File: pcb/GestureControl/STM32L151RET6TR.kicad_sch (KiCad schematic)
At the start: 33 parts, among them J10 EXTERN I2C, J11 Conn_01x02, J12 Conn_01x02, J17 Conn_01x01, J18 Conn_01x01, J19 Conn_01x01, J7 FTDI, J8 Conn_01x06, J9 UART, U6 STM32L151RETx, U7 STM32F401RETx, Y1 8MHz, Y2 32kHz

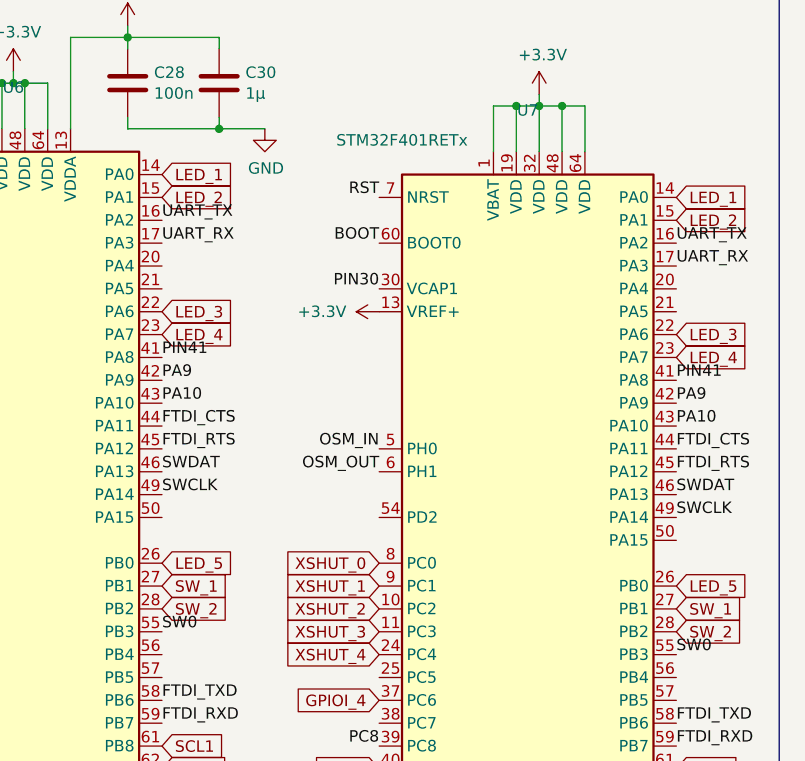
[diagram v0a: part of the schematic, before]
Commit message: add docs
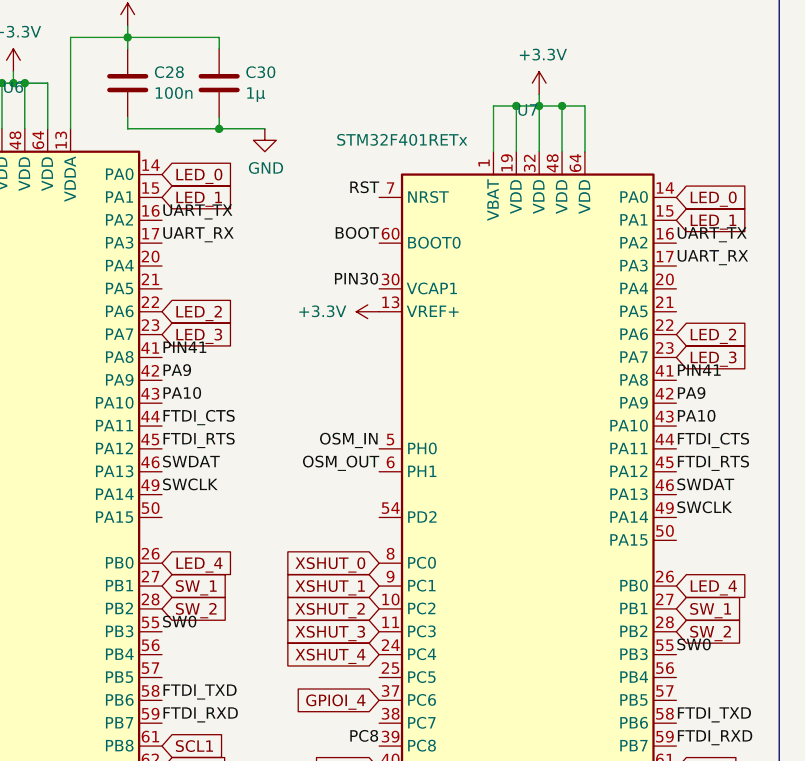
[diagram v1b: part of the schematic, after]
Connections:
- net LED_5 is gone; now on net LED_4: U6.26 (PB0), U7.26 (PB0)
- net LED_1: now also U6.15 (PA1), U7.15 (PA1); no longer U6.14 (PA0), U7.14 (PA0)
- net LED_2: now also U6.22 (PA6), U7.22 (PA6); no longer U6.15 (PA1), U7.15 (PA1)
- net LED_3: now also U6.23 (PA7), U7.23 (PA7); no longer U6.22 (PA6), U7.22 (PA6)
- net LED_4: no longer U6.23 (PA7), U7.23 (PA7)
- new net LED_0: U6.14 (PA0), U7.14 (PA0)
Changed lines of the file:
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@@
     )
   )
-  (global_label "LED_4" (shape input) (at 250.19 60.96 0) (fields_autoplaced)
-    (effects (font (size 1.27 1.27)) (justify left))
-    (property "Intersheet References" "${INTERSHEET_REFS}" (id 0) (at 0 0 0)
-      (effects (font (size 1.27 1.27)) hide)
-    )
-  )
-  (global_label "LED_1" (shape input) (at 193.04 40.64 0) (fields_autoplaced)
-    (effects (font (size 1.27 1.27)) (justify left))
-    (property "Intersheet References" "${INTERSHEET_REFS}" (id 0) (at 0 0 0)
-      (effects (font (size 1.27 1.27)) hide)
+  (global_label "LED_3" (shape input) (at 250.19 60.96 0) (fields_autoplaced)
+    (effects (font (size 1.27 1.27)) (justify left))
+    (property "Intersheet References" "${INTERSHEET_REFS}" (id 0) (at 258.1385 60.8806 0)
+      (effects (font (size 1.27 1.27)) (justify left) hide)
+    )
+  )
+  (global_label "LED_0" (shape input) (at 193.04 40.64 0) (fields_autoplaced)
+    (effects (font (size 1.27 1.27)) (justify left))
+    (property "Intersheet References" "${INTERSHEET_REFS}" (id 0) (at 200.9885 40.5606 0)
+      (effects (font (size 1.27 1.27)) (justify left) hide)
     )
   )
@@
     )
   )
-  (global_label "LED_2" (shape input) (at 193.04 43.18 0) (fields_autoplaced)
-    (effects (font (size 1.27 1.27)) (justify left))
-    (property "Intersheet References" "${INTERSHEET_REFS}" (id 0) (at 0 0 0)
-      (effects (font (size 1.27 1.27)) hide)
+  (global_label "LED_1" (shape input) (at 193.04 43.18 0) (fields_autoplaced)
+    (effects (font (size 1.27 1.27)) (justify left))
+    (property "Intersheet References" "${INTERSHEET_REFS}" (id 0) (at 200.9885 43.1006 0)
+      (effects (font (size 1.27 1.27)) (justify left) hide)
     )
   )
@@
     )
   )
-  (global_label "LED_2" (shape input) (at 250.19 45.72 0) (fields_autoplaced)
-    (effects (font (size 1.27 1.27)) (justify left))
-    (property "Intersheet References" "${INTERSHEET_REFS}" (id 0) (at 0 0 0)
-      (effects (font (size 1.27 1.27)) hide)
-    )
-  )
-  (global_label "LED_3" (shape input) (at 250.19 58.42 0) (fields_autoplaced)
-    (effects (font (size 1.27 1.27)) (justify left))
-    (property "Intersheet References" "${INTERSHEET_REFS}" (id 0) (at 0 0 0)
-      (effects (font (size 1.27 1.27)) hide)
+  (global_label "LED_1" (shape input) (at 250.19 45.72 0) (fields_autoplaced)
+    (effects (font (size 1.27 1.27)) (justify left))
+    (property "Intersheet References" "${INTERSHEET_REFS}" (id 0) (at 258.1385 45.6406 0)
+      (effects (font (size 1.27 1.27)) (justify left) hide)
+    )
+  )
+  (global_label "LED_2" (shape input) (at 250.19 58.42 0) (fields_autoplaced)
+    (effects (font (size 1.27 1.27)) (justify left))
+    (property "Intersheet References" "${INTERSHEET_REFS}" (id 0) (at 258.1385 58.3406 0)
+      (effects (font (size 1.27 1.27)) (justify left) hide)
     )
   )
@@
     )
   )
-  (global_label "LED_1" (shape input) (at 250.19 43.18 0) (fields_autoplaced)
-    (effects (font (size 1.27 1.27)) (justify left))
-    (property "Intersheet References" "${INTERSHEET_REFS}" (id 0) (at 0 0 0)
-      (effects (font (size 1.27 1.27)) hide)
+  (global_label "LED_0" (shape input) (at 250.19 43.18 0) (fields_autoplaced)
+    (effects (font (size 1.27 1.27)) (justify left))
+    (property "Intersheet References" "${INTERSHEET_REFS}" (id 0) (at 258.1385 43.1006 0)
+      (effects (font (size 1.27 1.27)) (justify left) hide)
     )
   )
@@
     )
   )
-  (global_label "LED_4" (shape input) (at 193.04 58.42 0) (fields_autoplaced)
-    (effects (font (size 1.27 1.27)) (justify left))
-    (property "Intersheet References" "${INTERSHEET_REFS}" (id 0) (at 0 0 0)
-      (effects (font (size 1.27 1.27)) hide)
+  (global_label "LED_3" (shape input) (at 193.04 58.42 0) (fields_autoplaced)
+    (effects (font (size 1.27 1.27)) (justify left))
+    (property "Intersheet References" "${INTERSHEET_REFS}" (id 0) (at 200.9885 58.3406 0)
+      (effects (font (size 1.27 1.27)) (justify left) hide)
     )
   )
@@
     )
   )
-  (global_label "LED_5" (shape input) (at 193.04 83.82 0) (fields_autoplaced)
-    (effects (font (size 1.27 1.27)) (justify left))
-    (property "Intersheet References" "${INTERSHEET_REFS}" (id 0) (at 0 0 0)
-      (effects (font (size 1.27 1.27)) hide)
+  (global_label "LED_4" (shape input) (at 193.04 83.82 0) (fields_autoplaced)
+    (effects (font (size 1.27 1.27)) (justify left))
+    (property "Intersheet References" "${INTERSHEET_REFS}" (id 0) (at 200.9885 83.7406 0)
+      (effects (font (size 1.27 1.27)) (justify left) hide)
     )
   )
@@
     )
   )
-  (global_label "LED_3" (shape input) (at 193.04 55.88 0) (fields_autoplaced)
-    (effects (font (size 1.27 1.27)) (justify left))
-    (property "Intersheet References" "${INTERSHEET_REFS}" (id 0) (at 0 0 0)
-      (effects (font (size 1.27 1.27)) hide)
-    )
-  )
-  (global_label "LED_5" (shape input) (at 250.19 86.36 0) (fields_autoplaced)
-    (effects (font (size 1.27 1.27)) (justify left))
-    (property "Intersheet References" "${INTERSHEET_REFS}" (id 0) (at 0 0 0)
-      (effects (font (size 1.27 1.27)) hide)
-    )
-  )
+  (global_label "LED_2" (shape input) (at 193.04 55.88 0) (fields_autoplaced)
+    (effects (font (size 1.27 1.27)) (justify left))
+    (property "Intersheet References" "${INTERSHEET_REFS}" (id 0) (at 200.9885 55.8006 0)
+      (effects (font (size 1.27 1.27)) (justify left) hide)
+    )
+  )
+  (global_label "LED_4" (shape input) (at 250.19 86.36 0) (fields_autoplaced)
+    (effects (font (size 1.27 1.27)) (justify left))
+    (property "Intersheet References" "${INTERSHEET_REFS}" (id 0) (at 258.1385 86.2806 0)
+      (effects (font (size 1.27 1.27)) (justify left) hide)
+    )
+  )
